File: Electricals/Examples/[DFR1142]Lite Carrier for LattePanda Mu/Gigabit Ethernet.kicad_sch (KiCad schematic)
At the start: 27 parts, among them J6 RJ45_RB1-125B8G1A, U6 RTL8111H-CG-RH, U7 ULC0524P, U8 ULC0524P, Y1 25MHz

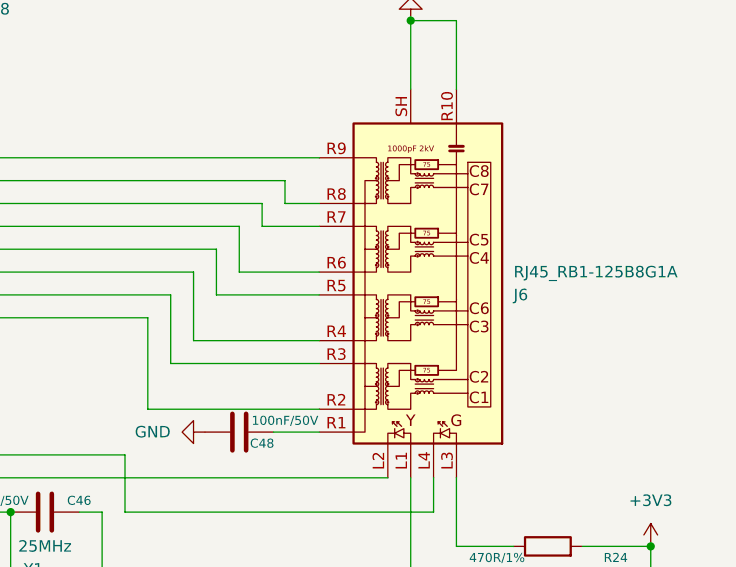
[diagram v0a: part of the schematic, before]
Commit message: new format
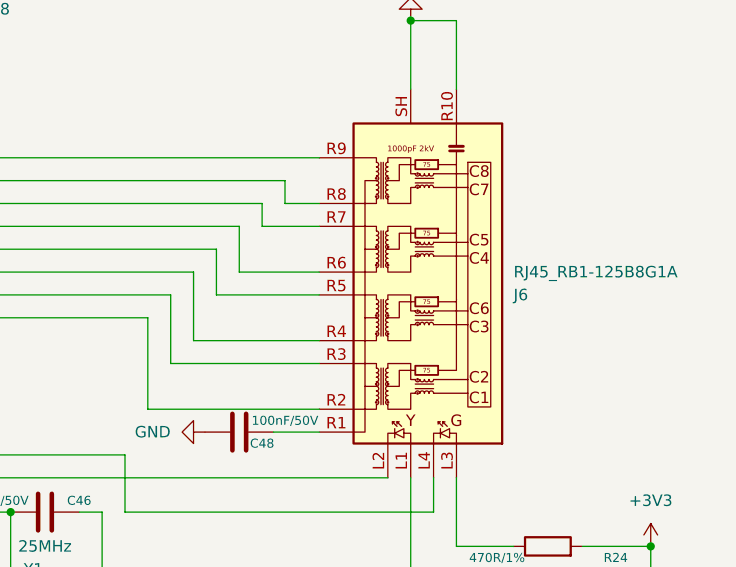
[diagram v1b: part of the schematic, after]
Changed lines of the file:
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@@
 (kicad_sch
-	(version 20231120)
+	(version 20250114)
 	(generator "eeschema")
-	(generator_version "8.0")
+	(generator_version "9.0")
 	(paper "A2")
 	(title_block
@@
 	(label "MDI0+"
 		(at 302.26 218.44 0)
-		(fields_autoplaced yes)
 		(effects
 			(font
@@
 	(label "MDI3-"
 		(at 275.59 139.7 0)
-		(fields_autoplaced yes)
 		(effects
 			(font
@@
 	(label "MDI1-"
 		(at 275.59 166.37 0)
-		(fields_autoplaced yes)
 		(effects
 			(font
@@
 	(label "MDI2-"
 		(at 302.26 205.74 0)
-		(fields_autoplaced yes)
 		(effects
 			(font
@@
 	(label "MDI3+"
 		(at 275.59 149.86 0)
-		(fields_autoplaced yes)
 		(effects
 			(font
@@
 	(label "MDI3+"
 		(at 302.26 203.2 0)
-		(fields_autoplaced yes)
 		(effects
 			(font
@@
 	(label "HSI+"
 		(at 243.84 233.68 0)
-		(fields_autoplaced yes)
 		(effects
 			(font
@@
 	(label "HSI-"
 		(at 243.84 231.14 0)
-		(fields_autoplaced yes)
 		(effects
 			(font
@@
 	(label "MDI1+"
 		(at 302.26 213.36 0)
-		(fields_autoplaced yes)
 		(effects
 			(font
@@
 	(label "MDI0-"
 		(at 334.01 166.37 0)
-		(fields_autoplaced yes)
 		(effects
 			(font
@@
 	(label "LED1_1000"
 		(at 302.26 233.68 0)
-		(fields_autoplaced yes)
 		(effects
 			(font
@@
 	(label "HSO+"
 		(at 243.84 241.3 0)
-		(fields_autoplaced yes)
 		(effects
 			(font
@@
 	(label "HSO-"
 		(at 243.84 238.76 0)
-		(fields_autoplaced yes)
 		(effects
 			(font
@@
 	(label "MDI0+"
 		(at 334.01 176.53 0)
-		(fields_autoplaced yes)
 		(effects
 			(font
@@
 	(label "MDI1-"
 		(at 302.26 210.82 0)
-		(fields_autoplaced yes)
 		(effects
 			(font
@@
 	(label "MDI3-"
 		(at 302.26 200.66 0)
-		(fields_autoplaced yes)
 		(effects
 			(font
@@
 	(label "MDI2+"
 		(at 302.26 208.28 0)
-		(fields_autoplaced yes)
 		(effects
 			(font
@@
 	(label "MDI1+"
 		(at 275.59 176.53 0)
-		(fields_autoplaced yes)
 		(effects
 			(font
@@
 	(label "LED2_ACT"
 		(at 302.26 236.22 0)
-		(fields_autoplaced yes)
 		(effects
 			(font
@@
 	(label "MDI2+"
 		(at 334.01 149.86 0)
-		(fields_autoplaced yes)
 		(effects
 			(font
@@
 	(label "LED0_100"
 		(at 302.26 231.14 0)
-		(fields_autoplaced yes)
 		(effects
 			(font
@@
 	(label "MDI2-"
 		(at 334.01 139.7 0)
-		(fields_autoplaced yes)
 		(effects
 			(font
@@
 	(label "MDI0-"
 		(at 302.26 215.9 0)
-		(fields_autoplaced yes)
 		(effects
 			(font
@@
 		(shape input)
 		(at 184.15 233.68 180)
-		(fields_autoplaced yes)
 		(effects
 			(font
@@
 		(shape input)
 		(at 184.15 251.46 180)
-		(fields_autoplaced yes)
 		(effects
 			(font
@@
 		(shape output)
 		(at 184.15 238.76 180)
-		(fields_autoplaced yes)
 		(effects
 			(font
@@
 		(shape output)
 		(at 184.15 241.3 180)
-		(fields_autoplaced yes)
 		(effects
 			(font
@@
 		(shape input)
 		(at 184.15 246.38 180)
-		(fields_autoplaced yes)
 		(effects
 			(font
@@
 		(shape input)
 		(at 184.15 231.14 180)
-		(fields_autoplaced yes)
 		(effects
 			(font
@@
 		(shape input)
 		(at 184.15 248.92 180)
-		(fields_autoplaced yes)
-		(effects
-			(font
+		(effects
+			(font
